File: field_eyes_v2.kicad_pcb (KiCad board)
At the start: 2 copper layers, 96 x 72 mm, 156 parts, among them J101 SOLAR 6V, J201 PROG, J202 OLED, J203 DHT22, J301 U.FL LTE, J302 SIM holder (TE 2199337-5), J303 MODEM USB (DNP), J401 SMT100 (V+ GND A B), J402 7-in-1 NPK (V+ GND A B), J403 VALVE coil, Q101 AO3401A, Q102 AO3401A, Q103 2N7002, Q104 FS8205, Q105 AO3401A, Q106 2N7002, Q107 AO3401A, Q108 2N7002, Q201 MMBT3904, Q202 MMBT3904, Q301 MMBT3904, Q302 MMBT3904, Q303 MMBT3904, Q304 MMBT3904, Q305 MMBT3904, Q306 MMBT3904, Q401 MMBT3904, Q402 MMBT3904, SW201 RESET, SW202 BOOT, U101 CN3791, U102 DW01A, U103 XC6220B331MR, U104 MT3608, U201 ESP32-WROOM-32D, U301 A7672S, U302 SMF05C, U401 SP3485EN, U402 SP3485EN, U403 MX1508, U404 L78L09

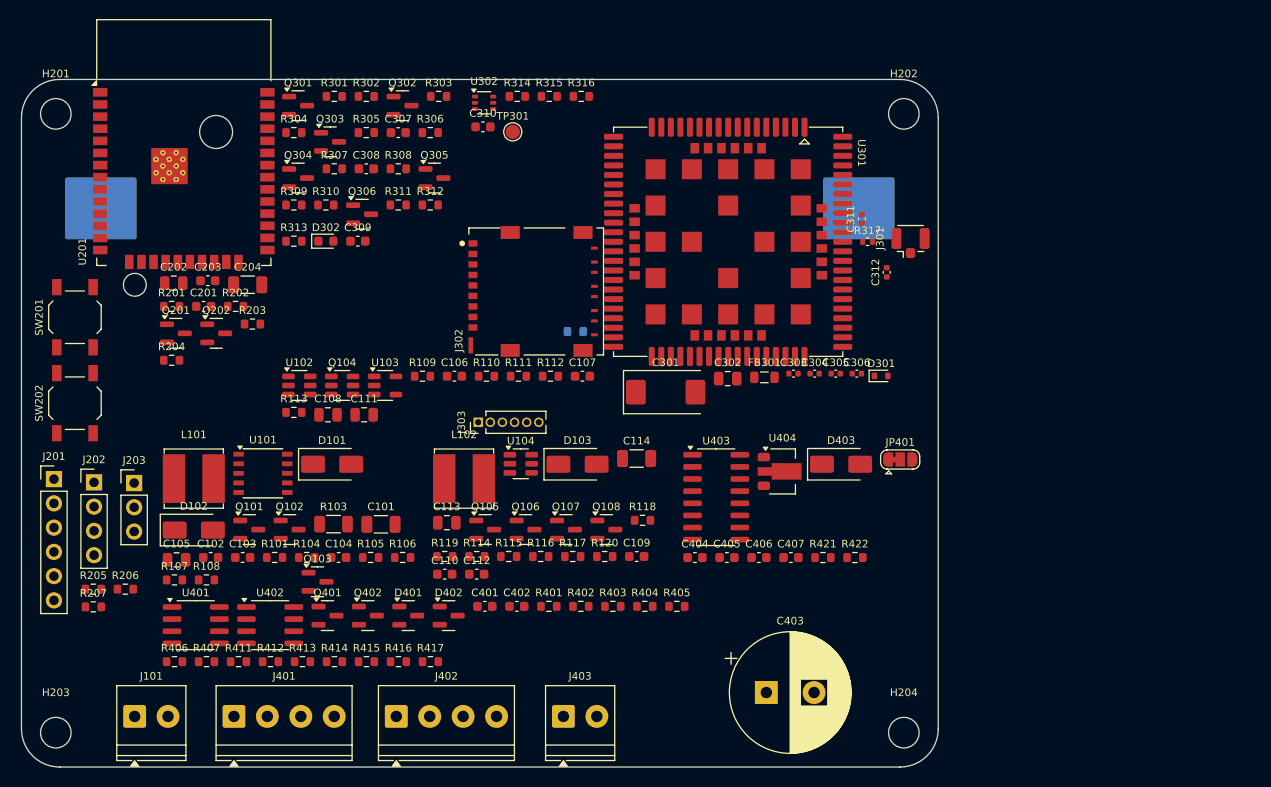
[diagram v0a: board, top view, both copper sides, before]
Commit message: repositioned ccomponents
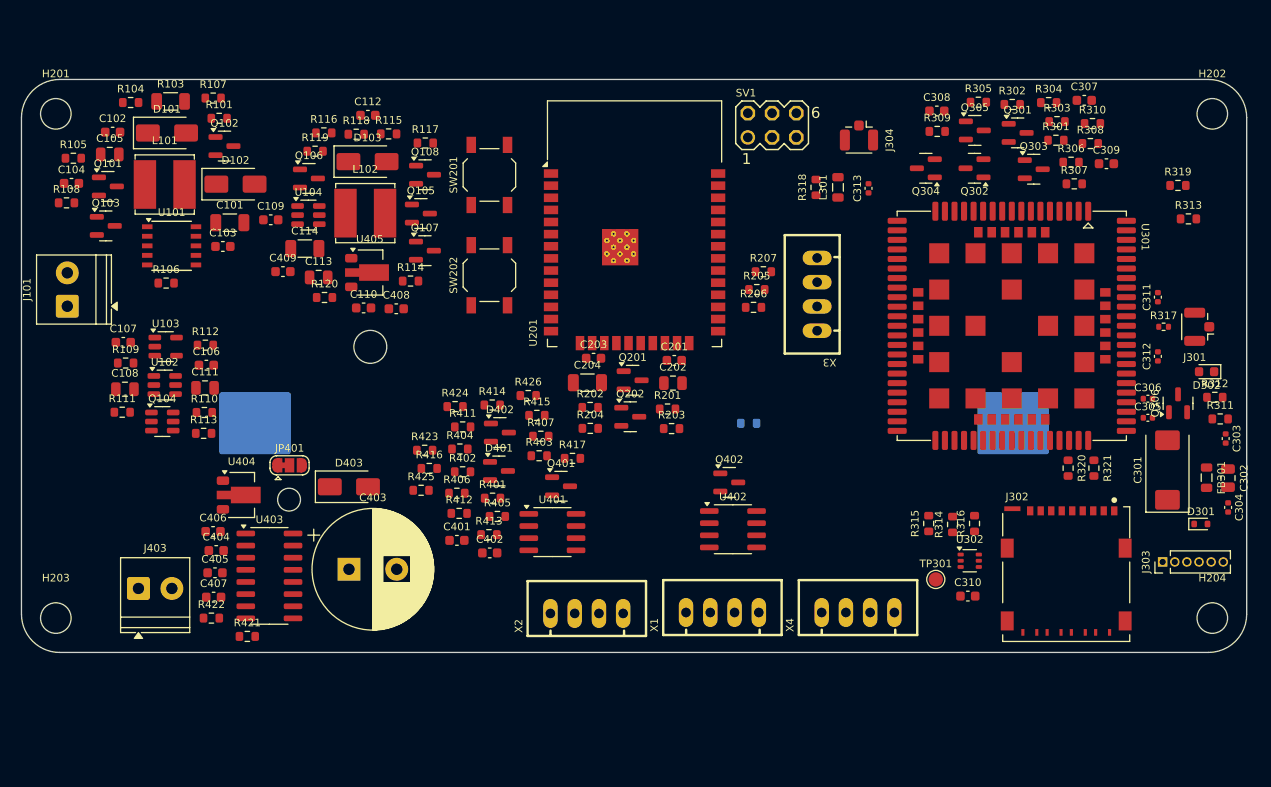
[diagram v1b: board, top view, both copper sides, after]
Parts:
- removed J201: PROG, Connector_PinHeader_2.54mm:PinHeader_1x06_P2.54mm_Vertical
- removed J202: OLED, Connector_PinHeader_2.54mm:PinHeader_1x04_P2.54mm_Vertical
- removed J203: DHT22, Connector_PinHeader_2.54mm:PinHeader_1x03_P2.54mm_Vertical
- removed J401: SMT100 (V+ GND A B), TerminalBlock_Phoenix:TerminalBlock_Phoenix_PT-1,5-4-3.5-H_1x04_P3.50mm_Horizontal
- removed J402: 7-in-1 NPK (V+ GND A B), TerminalBlock_Phoenix:TerminalBlock_Phoenix_PT-1,5-4-3.5-H_1x04_P3.50mm_Horizontal
- added C313: 33pF, Capacitor_SMD:C_0402_1005Metric, F.Cu at (174.8, 72.0)
- added C408: 330nF 25V, Capacitor_SMD:C_0603_1608Metric, F.Cu at (125.3, 84.6)
- added C409: 1uF, Capacitor_SMD:C_0603_1608Metric, F.Cu at (113.5, 80.7)
- added J304: U.FL GPS, Connector_Coaxial:U.FL_Hirose_U.FL-R-SMT-1_Vertical, F.Cu at (173.8, 66.5)
- added L301: 56nH, Inductor_SMD:L_0805_2012Metric, F.Cu at (171.6, 71.9)
- added R318: 0R, Resistor_SMD:R_0603_1608Metric, F.Cu at (169.3, 71.9)
- added R319: 10k, Resistor_SMD:R_0603_1608Metric, F.Cu at (207.2, 71.7)
- added R320: 1k, Resistor_SMD:R_0603_1608Metric, F.Cu at (195.7, 101.3)
- added R321: 1k, Resistor_SMD:R_0603_1608Metric, F.Cu at (198.4, 101.3)
- added R423: 3.3k, Resistor_SMD:R_0603_1608Metric, F.Cu at (128.3, 99.4)
- added R424: 6.8k, Resistor_SMD:R_0603_1608Metric, F.Cu at (131.5, 94.9)
- added R425: 3.3k, Resistor_SMD:R_0603_1608Metric, F.Cu at (127.9, 103.6)
- added R426: 6.8k, Resistor_SMD:R_0603_1608Metric, F.Cu at (139.2, 93.7)
- added SV1: PROG (as old SV1), field_eyes:MA03-2, F.Cu at (164.7, 65.4)
- added U405: L78L05, Package_TO_SOT_SMD:SOT-89-3, F.Cu at (122.6, 80.8)
- added X1: 7-in-1 NPK (A B 12V GND), field_eyes:JST_XH_04_LongPad, F.Cu at (159.5, 116.4)
- added X2: SMT100 (A B 12V GND), field_eyes:JST_XH_04_LongPad, F.Cu at (145.3, 116.5)
- added X3: OLED (3V3 GND SDA SCL), field_eyes:JST_XH_04_LongPad, F.Cu at (169.4, 83.1)
- added X4: DHT22 (NC 3V3 DATA GND), field_eyes:JST_XH_04_LongPad, F.Cu at (173.7, 116.4)
- U401, U402: value SP3485EN -> MAX485ESA+T
- moved R313 93.7 mm to (208.3, 75.2)
- moved D302 93.2 mm to (210.2, 91.2), turned to 180 degrees
- moved R311 88.9 mm to (211.6, 96.1)
- moved Q306 87.7 mm to (207.2, 94.5), turned to 90 degrees
- moved R312 84.6 mm to (211.1, 93.9)
- moved R310 80.7 mm to (198.2, 65.2)
- moved R304 79.1 mm to (193.7, 63.0)
- moved C309 78.8 mm to (199.7, 69.4)
- moved R207 78.5 mm to (163.8, 80.7)
- moved R307 77.5 mm to (196.3, 71.5)
- moved R205 76.2 mm to (163.1, 82.6)
- moved R301 75.7 mm to (194.4, 67.0)
- moved Q301 75.4 mm to (190.4, 66.2)
- moved Q303 73.7 mm to (192.1, 70.0)
- moved J303 73.2 mm to (205.6, 111.1)
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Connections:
- C401 pad 1: +3V3_SW -> +5V_SENS
- C402 pad 1: +3V3_SW -> +5V_SENS
- R402 pad 1: +3V3_SW -> +5V_SENS
- R403 pad 1: +3V3_SW -> +5V_SENS
- R412 pad 1: +3V3_SW -> +5V_SENS
- R413 pad 1: +3V3_SW -> +5V_SENS
- U301 pad P$116: (no net) -> +3V3
- U301 pad P$20: (no net) -> /MK_IN_3
- U301 pad P$49: (no net) -> /U3_RXD
- U301 pad P$50: (no net) -> /U3_TXD
- U301 pad P$90: (no net) -> /GPS_ANT
- U301 pad P$95: (no net) -> /GNSS_TXD
- U301 pad P$96: (no net) -> /GNSS_RXD
- U301 pad P$97: (no net) -> /VDD_1V8
- U301 pad P$98: (no net) -> /GNSS_PWRCTL
- U301 pad P$99: (no net) -> /VDD_2V8
- U401 pad 1: SMT_RX -> /RS1_RO
- U401 pad 8: +3V3_SW -> +5V_SENS
- U402 pad 1: NPK_RX -> /RS2_RO
- U402 pad 8: +3V3_SW -> +5V_SENS
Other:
- board size 96 x 72 mm -> 128.3 x 60 mm
